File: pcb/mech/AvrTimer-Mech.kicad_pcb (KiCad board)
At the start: 2 copper layers, 62.9 x 49.4 mm, 28 parts, among them J1 USB_B_Micro, Q1 BC846, SW1 SW_DIP_x01, SW2 SW_DIP_x01, SW3 SW_DIP_x01, SW4 SW_DPDT_x2, SW5 SW_DIP_x02, U1 L7805

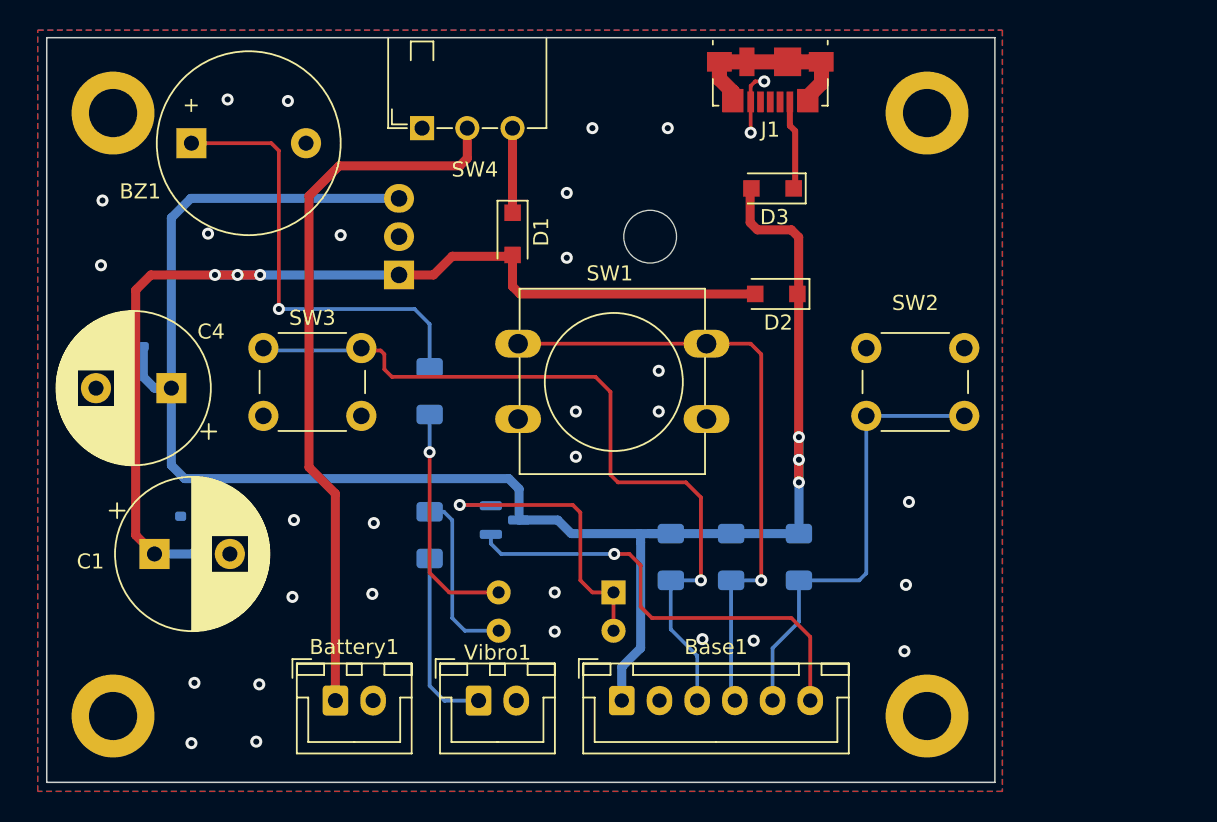
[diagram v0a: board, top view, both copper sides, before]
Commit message: Update after Alexander's review
Change-Id: Ia4ad441f5e963f780b6a0a3a3c0dc55fa8eb64d7
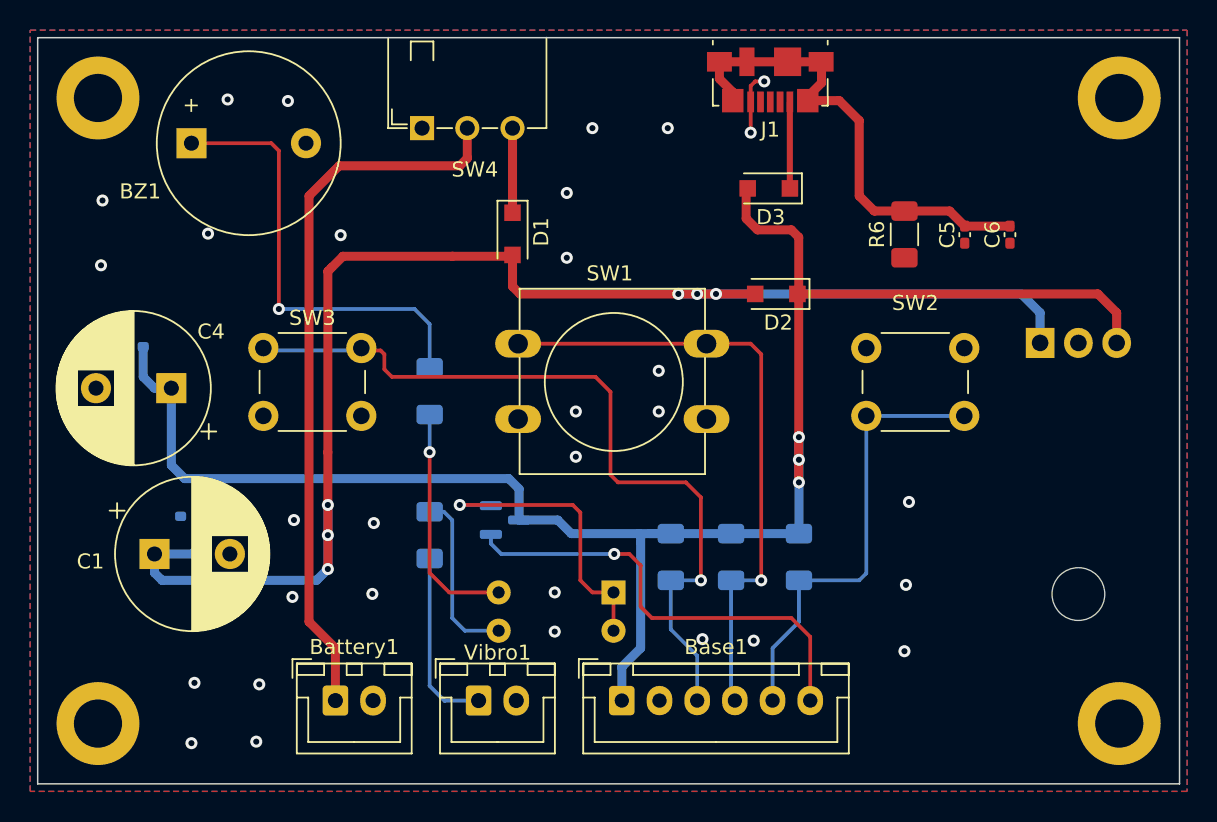
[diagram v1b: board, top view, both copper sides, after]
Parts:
- added C5: C, Capacitor_SMD:C_0402_1005Metric_Pad0.74x0.62mm_HandSolder, F.Cu at (144.5, 69.1)
- added C6: C, Capacitor_SMD:C_0402_1005Metric_Pad0.74x0.62mm_HandSolder, F.Cu at (147.5, 69.1)
- added R6: R, Resistor_SMD:R_1206_3216Metric_Pad1.30x1.75mm_HandSolder, F.Cu at (140.5, 69.0)
- moved U1 42.8 mm to (149.5, 76.2), turned to 0 degrees
- moved ? 12.8 mm to (154.8, 60.0)
- moved ? 12.8 mm to (154.8, 101.5)
- moved ? 1.41 mm to (87.0, 60.0)
- moved ? 1.12 mm to (87.0, 101.5)
- moved D3 0.25 mm to (131.5, 66.0)
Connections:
- J1 pad 6: unconnected-(J1-Pad6) -> Net-(J1-Pad6)
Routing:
- net Net-(J1-Pad6): track 0.00 -> 32.4 mm
- net Net-(C1-Pad1): track 70.3 -> 99.8 mm, vias 3 -> 6
- net unconnected-(J1-Pad6): track 12.7 -> 0.00 mm
- net VCC: track 122.5 -> 119.5 mm
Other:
- board size 62.9 x 49.4 mm -> 75.8 x 49.5 mm
